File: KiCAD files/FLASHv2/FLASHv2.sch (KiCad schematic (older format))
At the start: 14 parts, among them J1 card addr, J2 Power Bus, J3 Signal Bus, J4 IDE connector, U1 74LS04, U2 74LS85, U3 74LS245, U4 74LS245

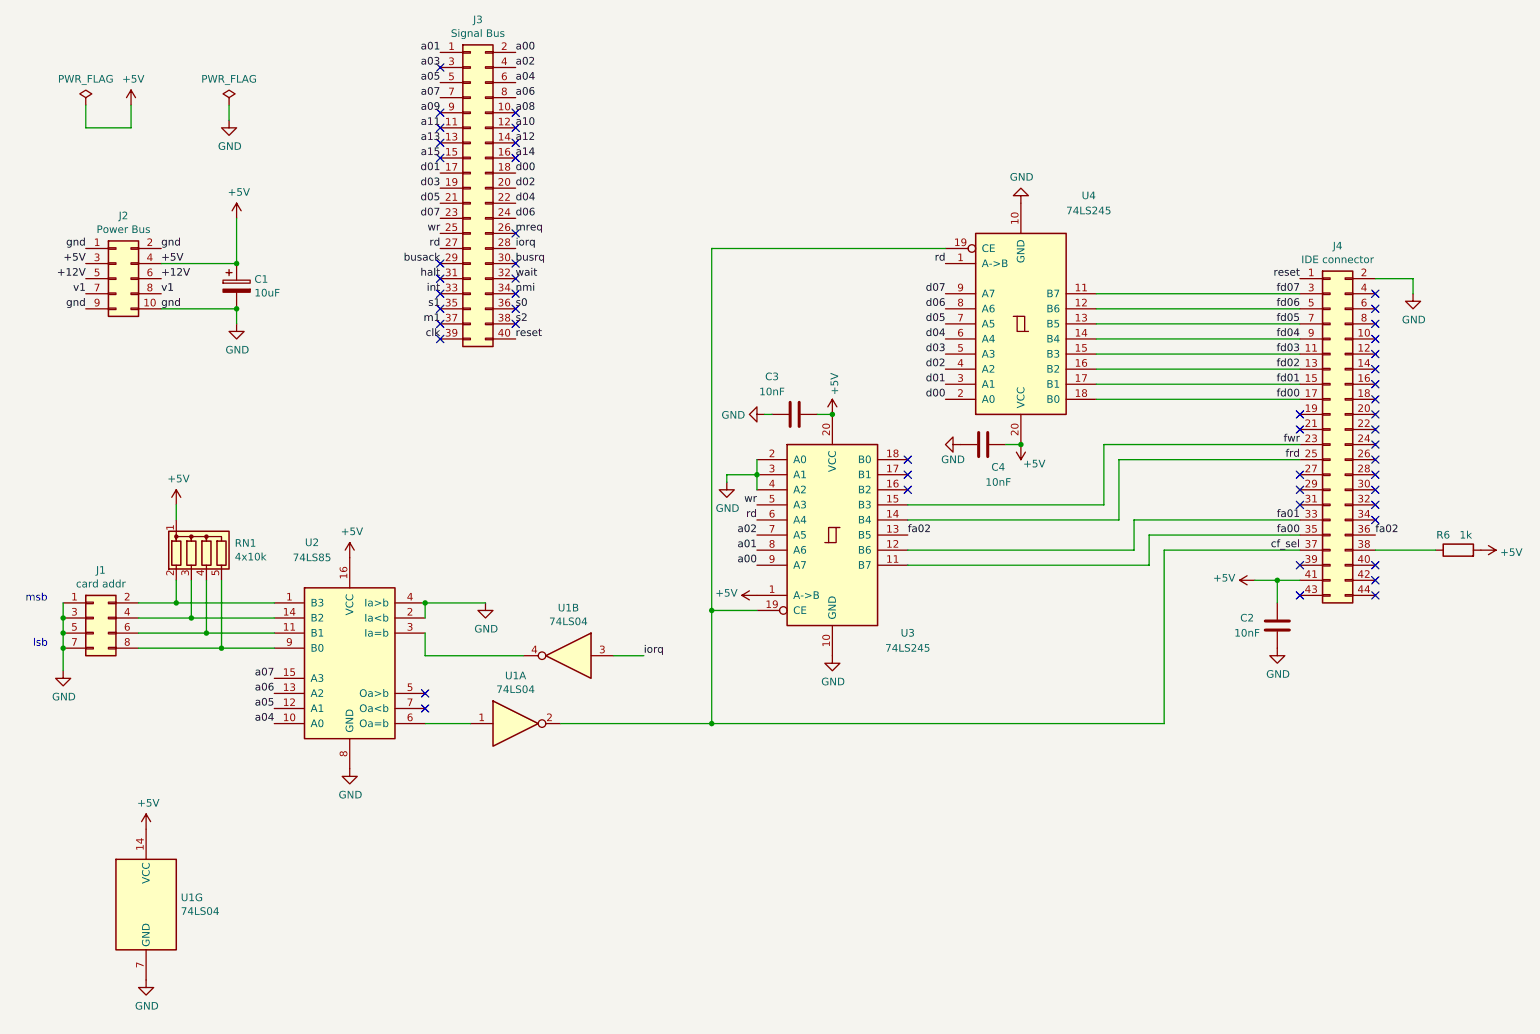
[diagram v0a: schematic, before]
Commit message: home
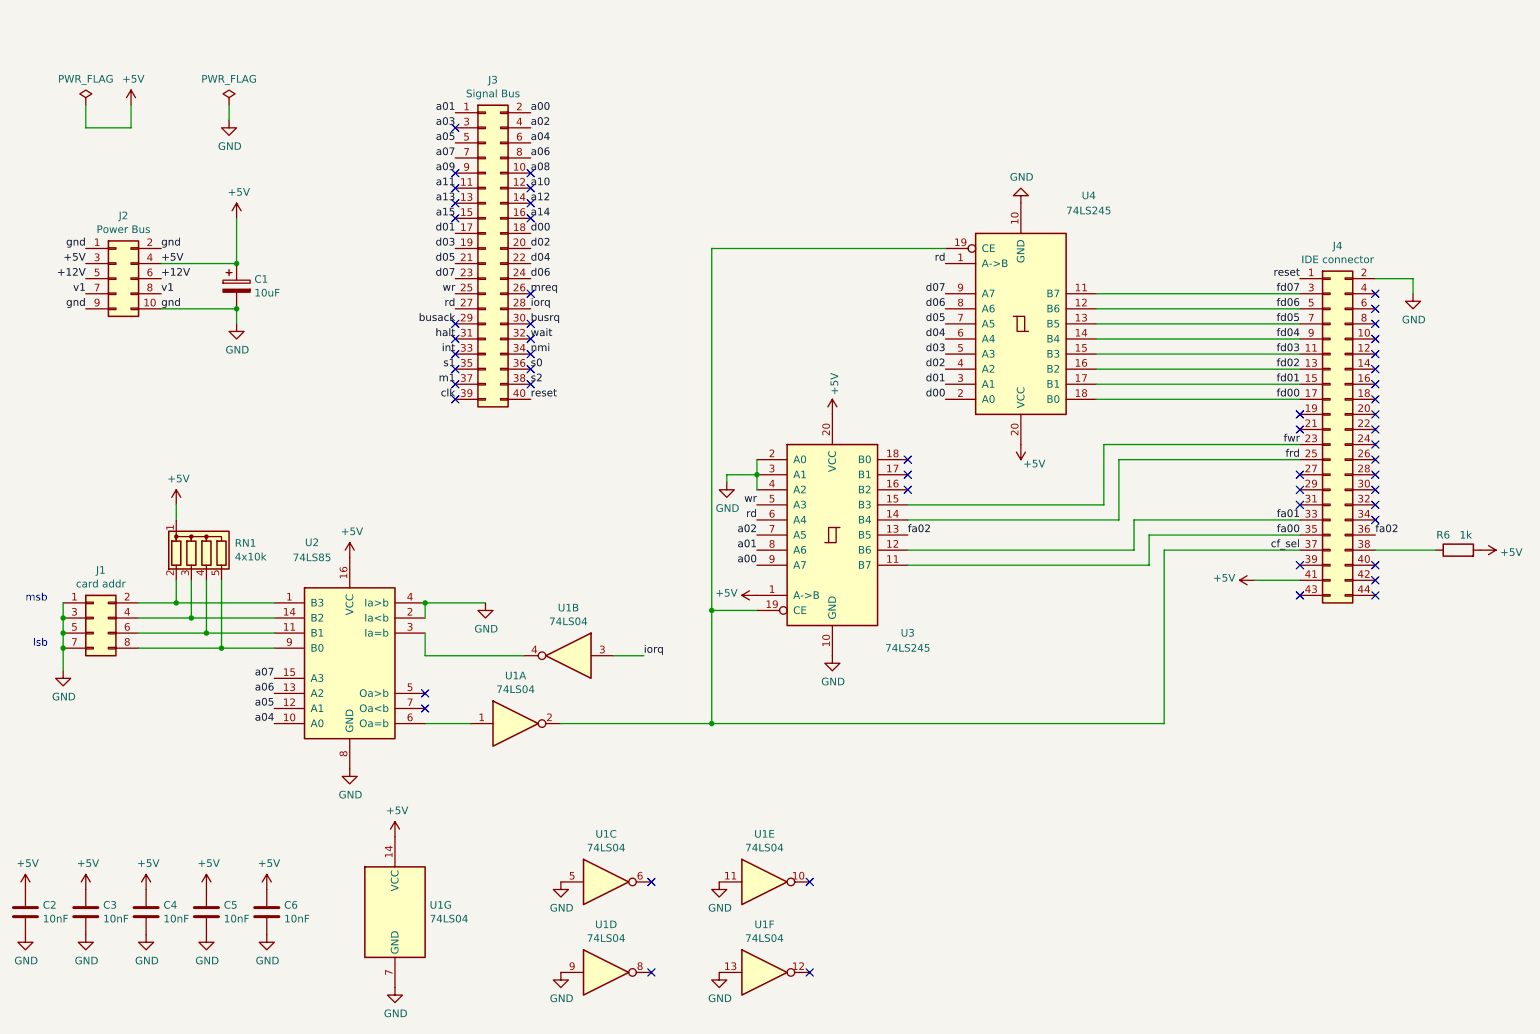
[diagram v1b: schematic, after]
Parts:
- added C5, C6: 10nF, Capacitor_THT:C_Disc_D3.8mm_W2.6mm_P2.50mm, symbol Device:C
- added unit 3 of U1
- added unit 4 of U1
- added unit 5 of U1
- added unit 6 of U1
- C1: footprint (none) -> Capacitor_THT:CP_Radial_D5.0mm_P2.50mm
- C2, C3, C4: footprint (none) -> Capacitor_THT:C_Disc_D3.8mm_W2.6mm_P2.50mm
- J1: footprint (none) -> Connector_PinHeader_2.54mm:PinHeader_2x04_P2.54mm_Vertical
- J2: footprint (none) -> Connector_PinHeader_2.54mm:PinHeader_2x05_P2.54mm_Vertical
- J3: footprint (none) -> Connector_PinHeader_2.54mm:PinHeader_2x20_P2.54mm_Vertical
- J4: footprint (none) -> Connector_PinHeader_2.00mm:PinHeader_2x22_P2.00mm_Vertical
- R6: footprint (none) -> Resistor_THT:R_Axial_DIN0207_L6.3mm_D2.5mm_P10.16mm_Horizontal
- U1: footprint (none) -> Package_DIP:DIP-14_W7.62mm_Socket_LongPads
- U2: footprint (none) -> Package_DIP:DIP-16_W7.62mm_Socket_LongPads
- U3, U4: footprint (none) -> Package_DIP:DIP-20_W7.62mm_Socket_LongPads
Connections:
- net +5V: now also C5.1, C6.1
- net GND: now also C5.2, C6.2, U1.11, U1.13, U1.5, U1.9
- no-connect marks 52 -> 56
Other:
- moved on the sheet: J3, U1G
